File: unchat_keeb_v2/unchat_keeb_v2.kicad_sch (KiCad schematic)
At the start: 21 parts, among them J1 RJ45, J51 RJ45

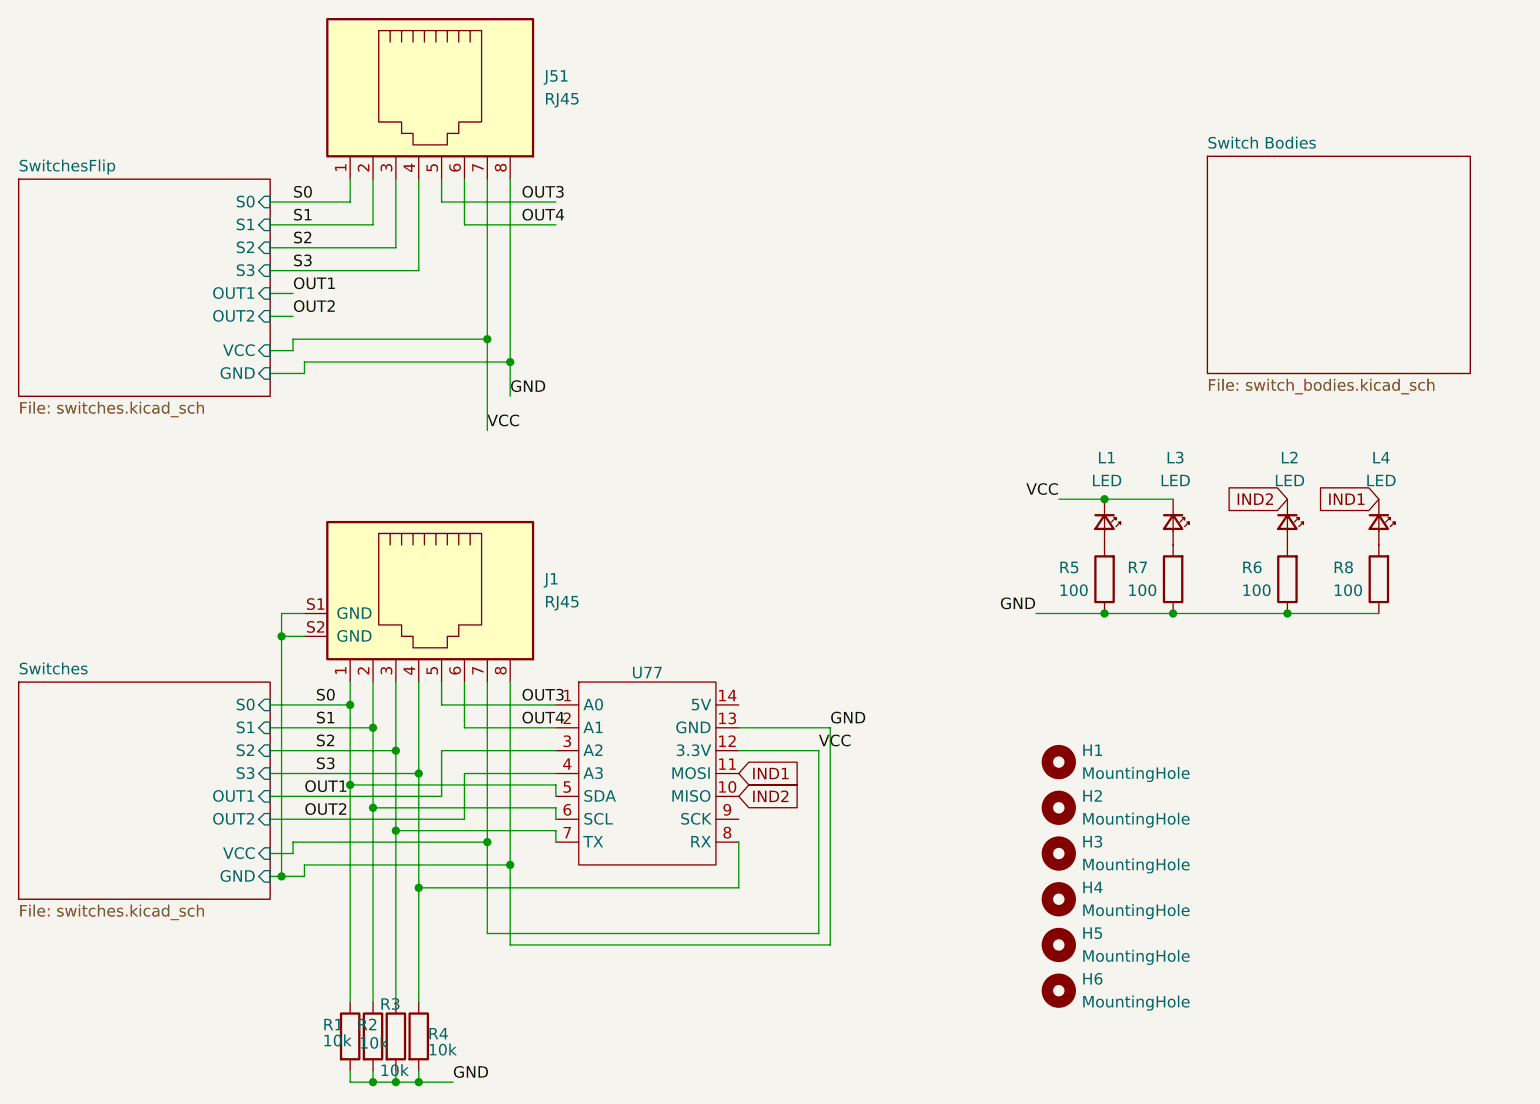
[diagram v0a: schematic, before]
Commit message: readme: Added with many images and a snippet of the timelapse
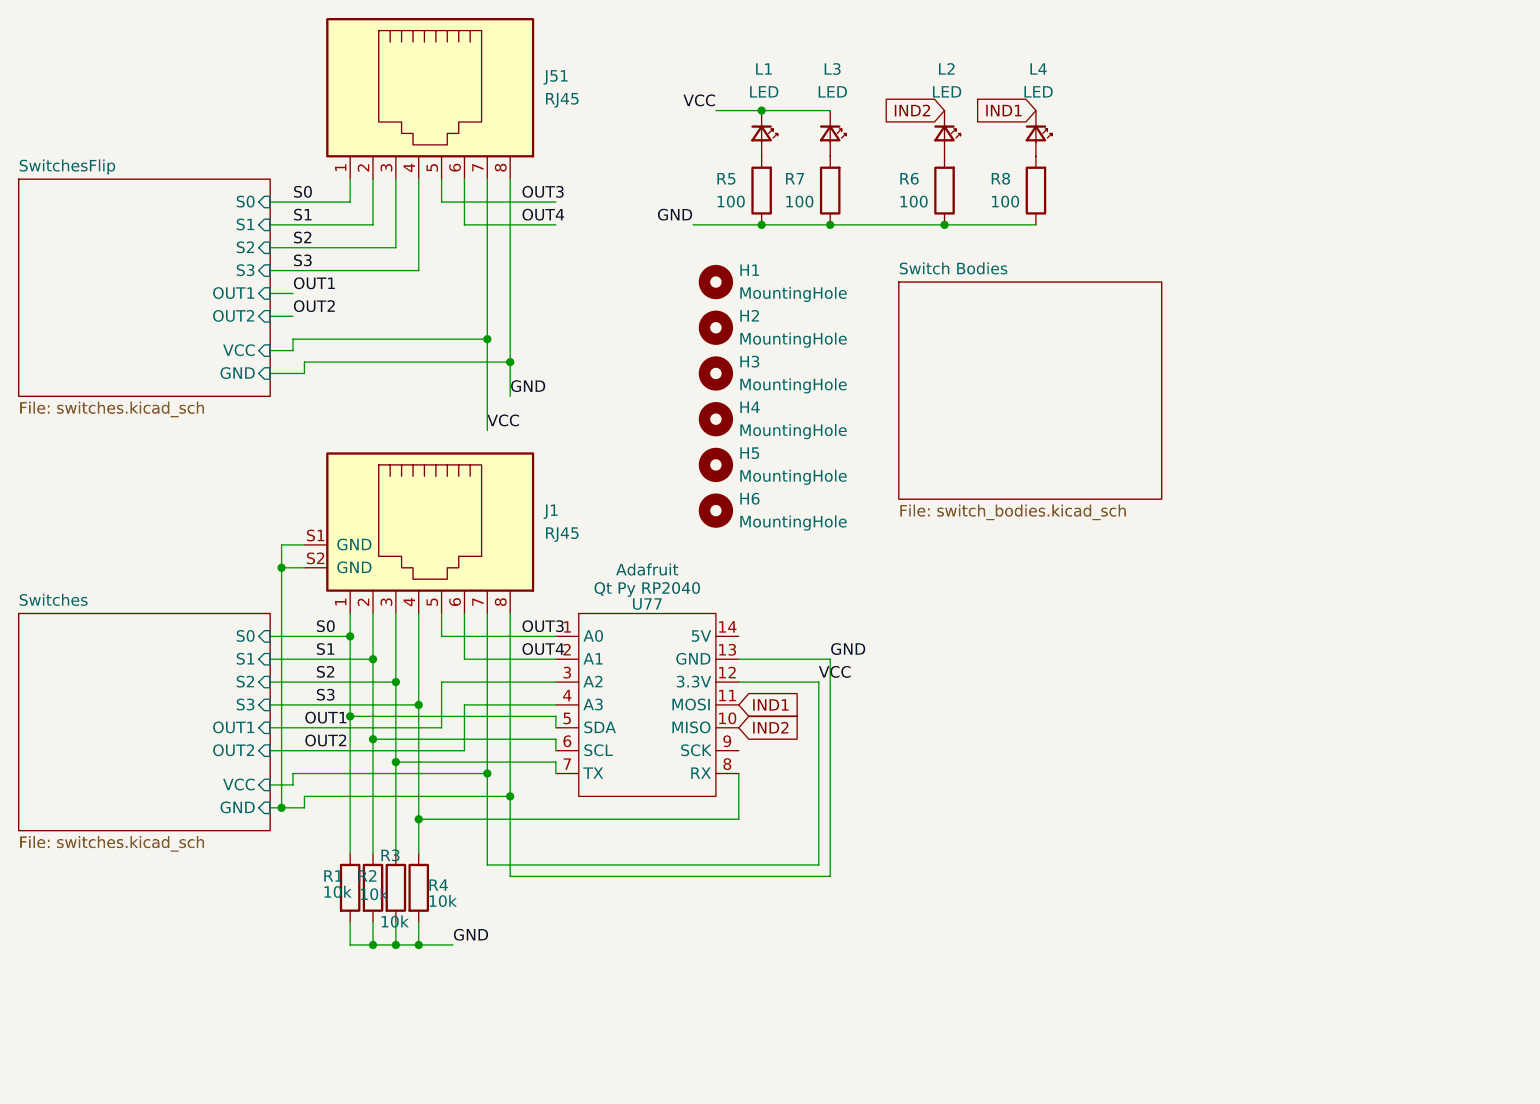
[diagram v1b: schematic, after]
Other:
- note added: "Adafruit Qt Py RP2040"
- moved on the sheet: H1, H2, H3, H4, H5, H6, J1, L1, L2, L3, L4, R1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
